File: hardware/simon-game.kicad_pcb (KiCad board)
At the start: 2 copper layers, 50 x 50 mm, 17 parts, among them SW1 SW_Push, SW2 SW_Push, SW3 SW_Push, SW4 SW_Push, U1 ATtiny402-SS

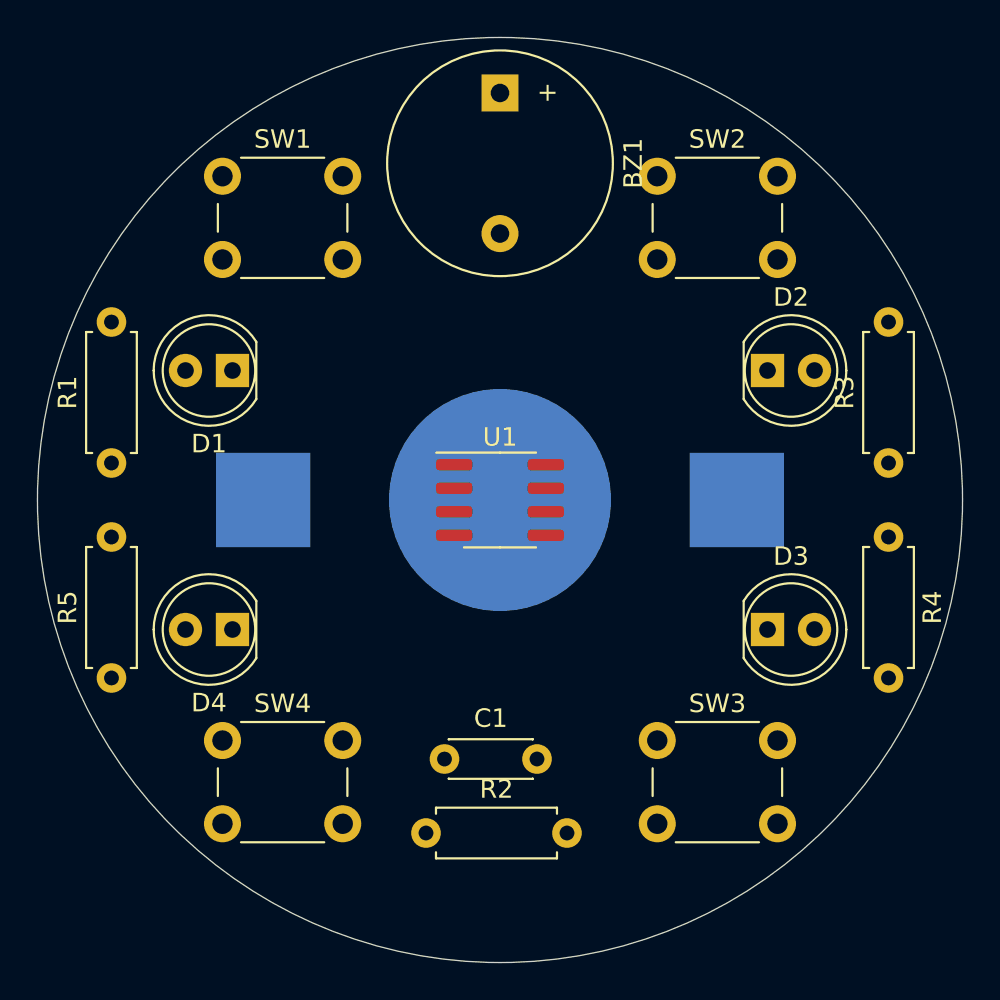
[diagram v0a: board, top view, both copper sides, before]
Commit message: Working on PCB
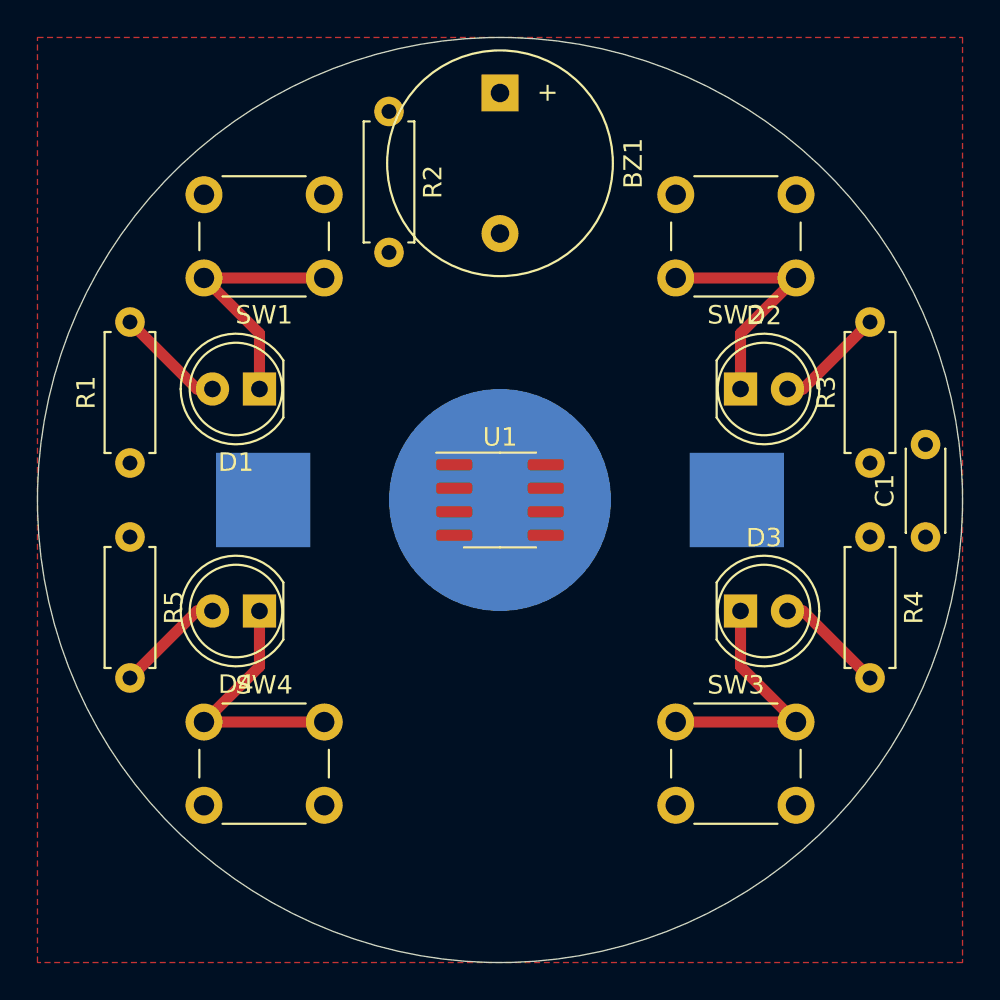
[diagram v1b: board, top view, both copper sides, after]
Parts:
- moved R2 39.1 mm to (144.0, 72.0), turned to 270 degrees
- moved C1 28.6 mm to (173.0, 95.0), turned to 90 degrees
- moved SW2 9.30 mm to (166.0, 81.0), turned to 180 degrees
- moved SW1 7.78 mm to (140.5, 81.0), turned to 180 degrees
- moved R5 7.69 mm to (130.0, 95.0), turned to 270 degrees
- moved D1 1.77 mm to (137.0, 87.0)
- moved D2 1.77 mm to (163.0, 87.0)
- moved D3 1.77 mm to (163.0, 99.0)
- moved D4 1.77 mm to (137.0, 99.0)
- moved SW3 1.41 mm to (159.5, 105.0)
- moved SW4 1.41 mm to (134.0, 105.0)
- moved R1 1.00 mm to (130.0, 91.0)
- moved R3 1.00 mm to (170.0, 91.0)
- moved R4 1.00 mm to (170.0, 95.0)
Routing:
- net Net-(D4-Pad1): track 0.00 -> 13.7 mm
- net Net-(D3-Pad1): track 0.00 -> 13.7 mm
- net Net-(D2-Pad1): track 0.00 -> 13.7 mm
- net Net-(D1-Pad1): track 0.00 -> 13.7 mm
- net Net-(D4-Pad2): track 0.00 -> 5.96 mm
- net Net-(D3-Pad2): track 0.00 -> 5.96 mm
- net Net-(D2-Pad2): track 0.00 -> 5.96 mm
- net Net-(D1-Pad2): track 0.00 -> 5.96 mm
- added copper zone on F.Cu, net GND

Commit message: Finished PCB
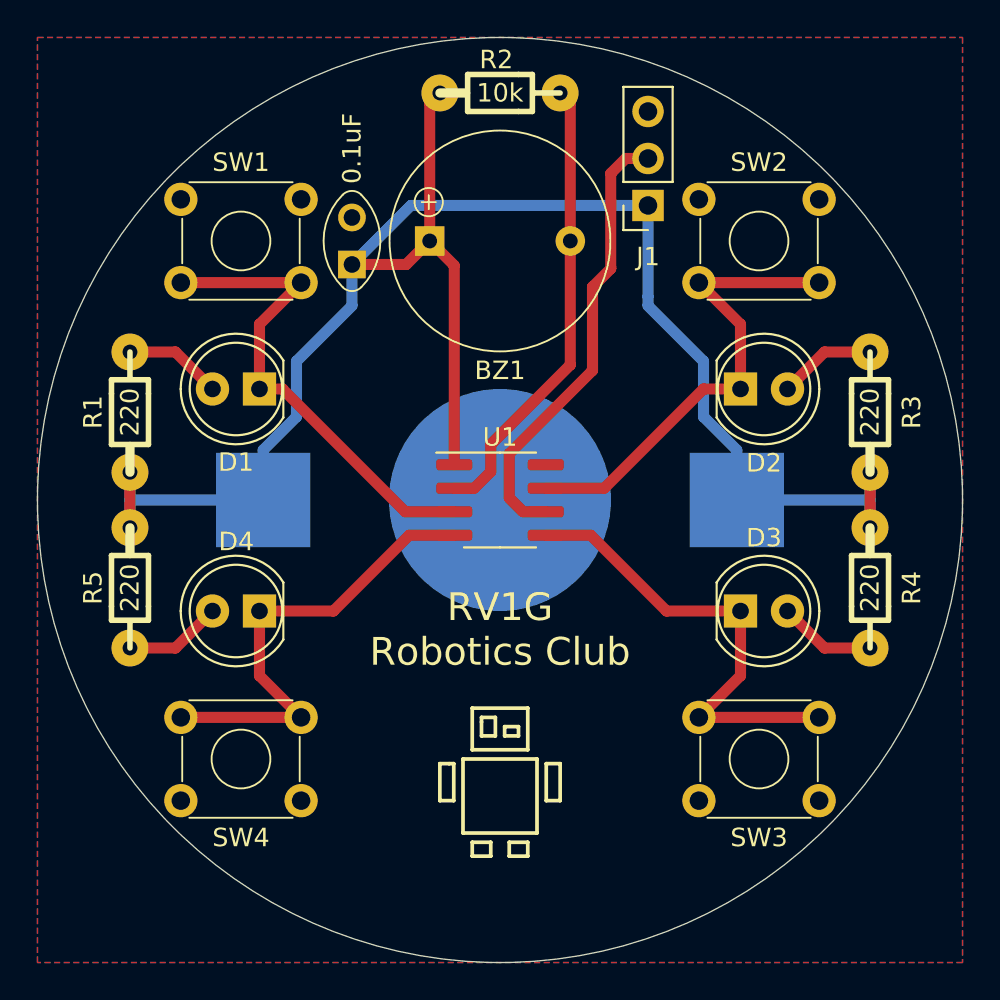
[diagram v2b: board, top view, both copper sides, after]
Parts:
- added J1: Conn_01x03_Male, Connector_PinSocket_2.54mm:PinSocket_1x03_P2.54mm_Vertical, F.Cu at (158.0, 77.1)
- BZ1: footprint Buzzer_Beeper:Buzzer_12x9.5RM7.6 -> ingus_electromechanics:Beeper_12xx
- C1: footprint Capacitor_THT:C_Disc_D4.3mm_W1.9mm_P5.00mm -> janis:CE-2mm54
- R1, R2, R3, R4, R5: footprint Resistor_THT:R_Axial_DIN0207_L6.3mm_D2.5mm_P7.62mm_Horizontal -> janis:R_W8_THT_Hor
- SW1, SW2, SW3: footprint Button_Switch_THT:SW_PUSH_6mm -> ingus_electromechanics:6x6_SPST
- SW4: value SW_Push -> TACTILE_SW_4Pin; footprint Button_Switch_THT:SW_PUSH_6mm -> ingus_electromechanics:6x6_SPST
- moved C1 34.9 mm to (142.0, 79.0)
- moved BZ1 8.00 mm to (150.0, 79.0), turned to 0 degrees
- moved R2 6.08 mm to (150.0, 71.0), turned to 0 degrees
- moved SW1 4.92 mm to (136.0, 79.0)
- moved SW3 4.92 mm to (164.0, 107.0)
- moved SW2 2.83 mm to (164.0, 79.0)
- moved SW4 2.83 mm to (136.0, 107.0)
- moved R1 2.75 mm to (130.0, 88.2)
- moved R3 2.75 mm to (170.0, 88.2)
- moved R4 2.75 mm to (170.0, 97.8)
- moved R5 2.75 mm to (130.0, 97.8)
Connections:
- SW1 pad 2: GND -> Net-(D1-Pad1)
- SW2 pad 2: GND -> Net-(D2-Pad1)
- SW3 pad 2: GND -> Net-(D3-Pad1)
- SW4 pad 2: GND -> Net-(D4-Pad1)
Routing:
- net Net-(BAT1-Pad1): track 0.00 -> 101.9 mm
- net /BUZZER: track 0.00 -> 24.8 mm
- net /RESET_UPDI: track 0.00 -> 24.4 mm
- net Net-(D1-Pad1): track 13.7 -> 26.5 mm
- net Net-(D2-Pad1): track 13.7 -> 25.9 mm
- net Net-(D4-Pad1): track 13.7 -> 25.4 mm
- net Net-(D3-Pad1): track 13.7 -> 25.4 mm
- net Net-(D4-Pad2): track 5.96 -> 5.29 mm
- net Net-(D3-Pad2): track 5.96 -> 5.29 mm
- net Net-(D2-Pad2): track 5.96 -> 5.29 mm
- net Net-(D1-Pad2): track 5.96 -> 5.29 mm
- added copper zone on B.Cu, net GND
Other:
- board text added: "2019"
- board text added: "RV1G Robotics Club"
- board text added: "Simon Game"
